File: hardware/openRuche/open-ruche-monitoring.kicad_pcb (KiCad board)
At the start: 2 copper layers, 139.4 x 98.4 mm, 29 parts, among them J1 HX711, J10 MMA8451, J11 CONN ALIM, J12 BAT ESP32, J2 DHT22_EXT, J3 DHT22_INT, J4 SONDE_TEMP_1, J5 SONDE_TEMP_2, J6 LUX, J7 LORA, J8 ARDUINO, J9 XIAO, U1 uPesy ESP32 Wroom Low Power D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, U2 S7V8F3, U3 S7V8F5

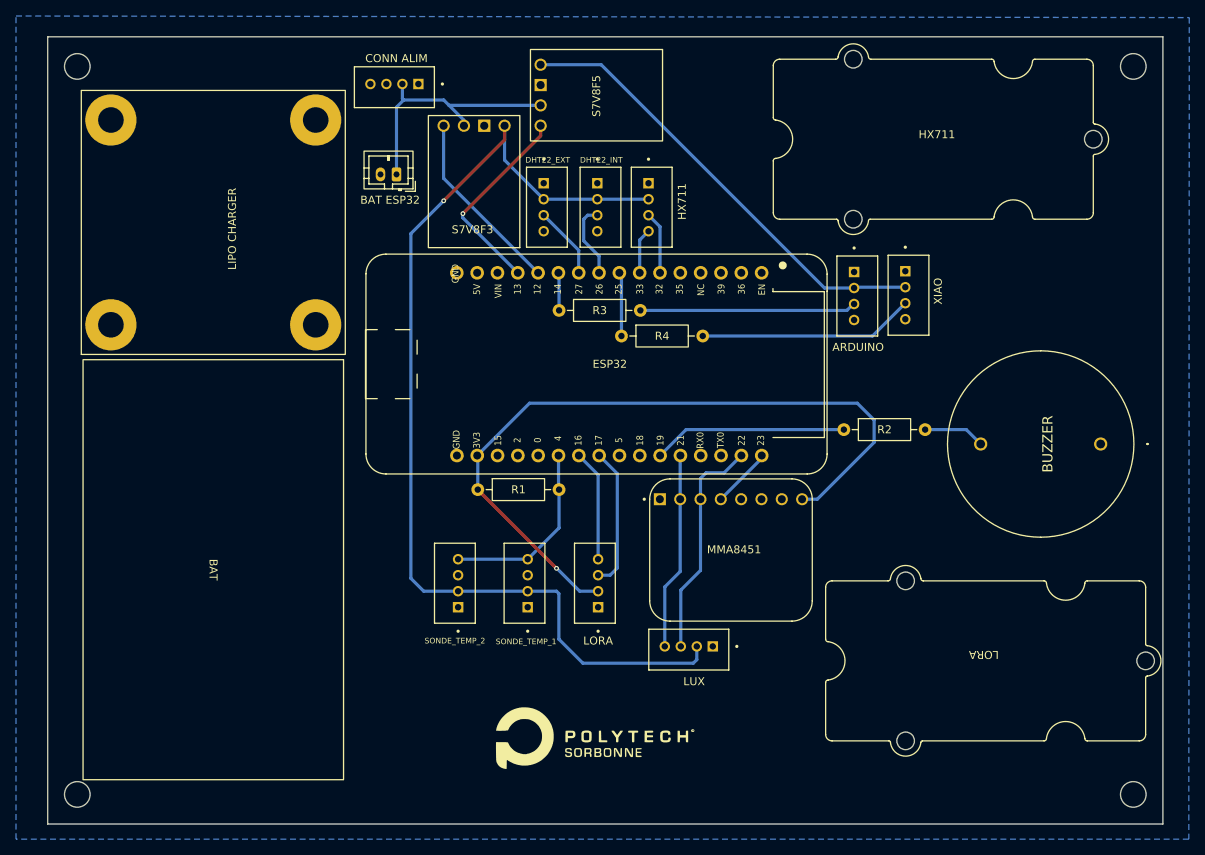
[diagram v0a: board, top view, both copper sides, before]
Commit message: hw(pcb) gerber files
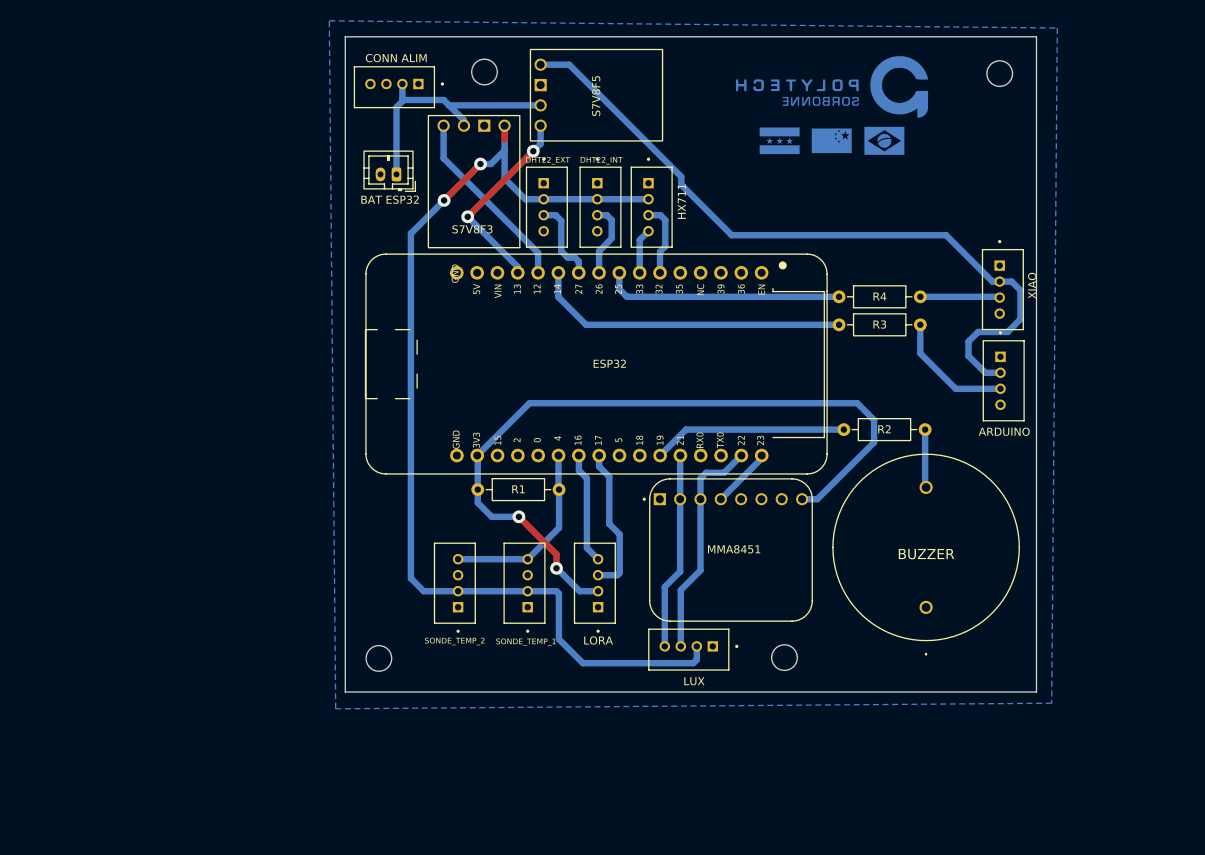
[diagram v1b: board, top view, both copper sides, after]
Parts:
- removed BAT: lipo_bat, battery:lipo_bat
- removed LIPO_CHARGER: LIPO CHARGER, lipo_charger:DFR0264
- removed LORA: lora_module, lora_grove:lora_module
- removed the REF** at (174.4, 55.8)
- added G***: LOGO, battery:brasil, F.Cu at (186.4, 56.0)
- added G***: LOGO, battery:syria, F.Cu at (173.5, 56.0)
- added G***: LOGO, battery:china, F.Cu at (179.6, 56.0)
- moved G*** 86.8 mm to (180.3, 49.3)
- moved REF** 50.9 mm to (136.4, 47.4)
- moved REF** 46.8 mm to (173.9, 120.6)
- moved REF** 41.4 mm to (123.2, 120.7)
- moved R3 35.0 mm to (180.7, 79.0)
- moved BUZZER 29.9 mm to (191.6, 114.3), turned to 0 degrees
- moved R4 27.6 mm to (180.7, 75.5)
- moved J8 21.1 mm to (200.9, 86.0)
- moved REF** 16.7 mm to (200.8, 47.6)
- moved J9 11.8 mm to (200.8, 74.6)
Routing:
- net /TX_ARDUINO: track 4.73 -> 39.6 mm
- net /+5V_REG: track 57.2 -> 90.2 mm
- net /TX_XIAO: track 8.01 -> 30.3 mm
- net Net-(J9-SIG1): track 27.0 -> 9.96 mm
- net Net-(J8-SIG1): track 27.1 -> 15.4 mm
- net /+3.3V: track 92.6 -> 94.6 mm, vias 1 -> 2
- net /DOUT: track 7.80 -> 9.22 mm
- net /DATA_DHT22_EXT: track 9.01 -> 10.4 mm
- net /+3.3V_REG: track 131.1 -> 132.0 mm, vias 1 -> 2
- net /RX_LORA: track 17.8 -> 18.5 mm
- net /EN_5V_REG: track 25.3 -> 24.8 mm, vias 1 -> 2
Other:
- board size 139.4 x 98.4 mm -> 86.4 x 81.9 mm
